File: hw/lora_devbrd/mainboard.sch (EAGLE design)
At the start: 15 parts, among them IC1 FT232RL, U1 RHF78-052

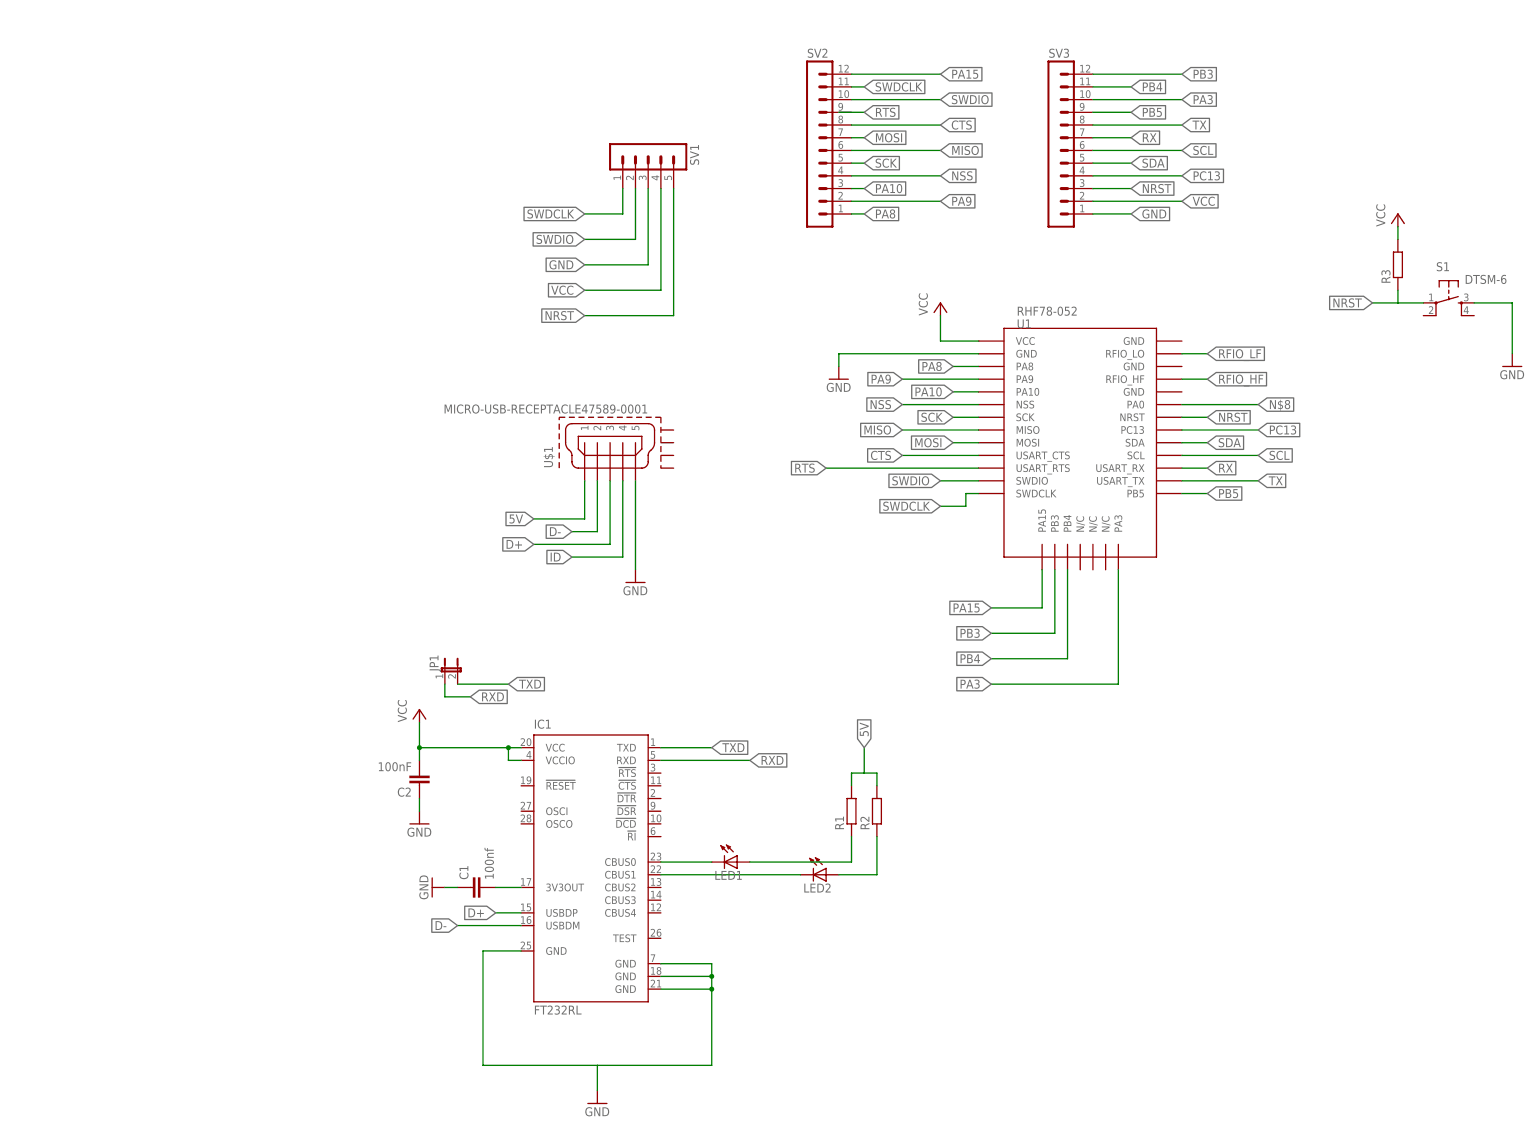
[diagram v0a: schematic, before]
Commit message: Adds LM1117
TODO:
            * trace board
            * check, check, check
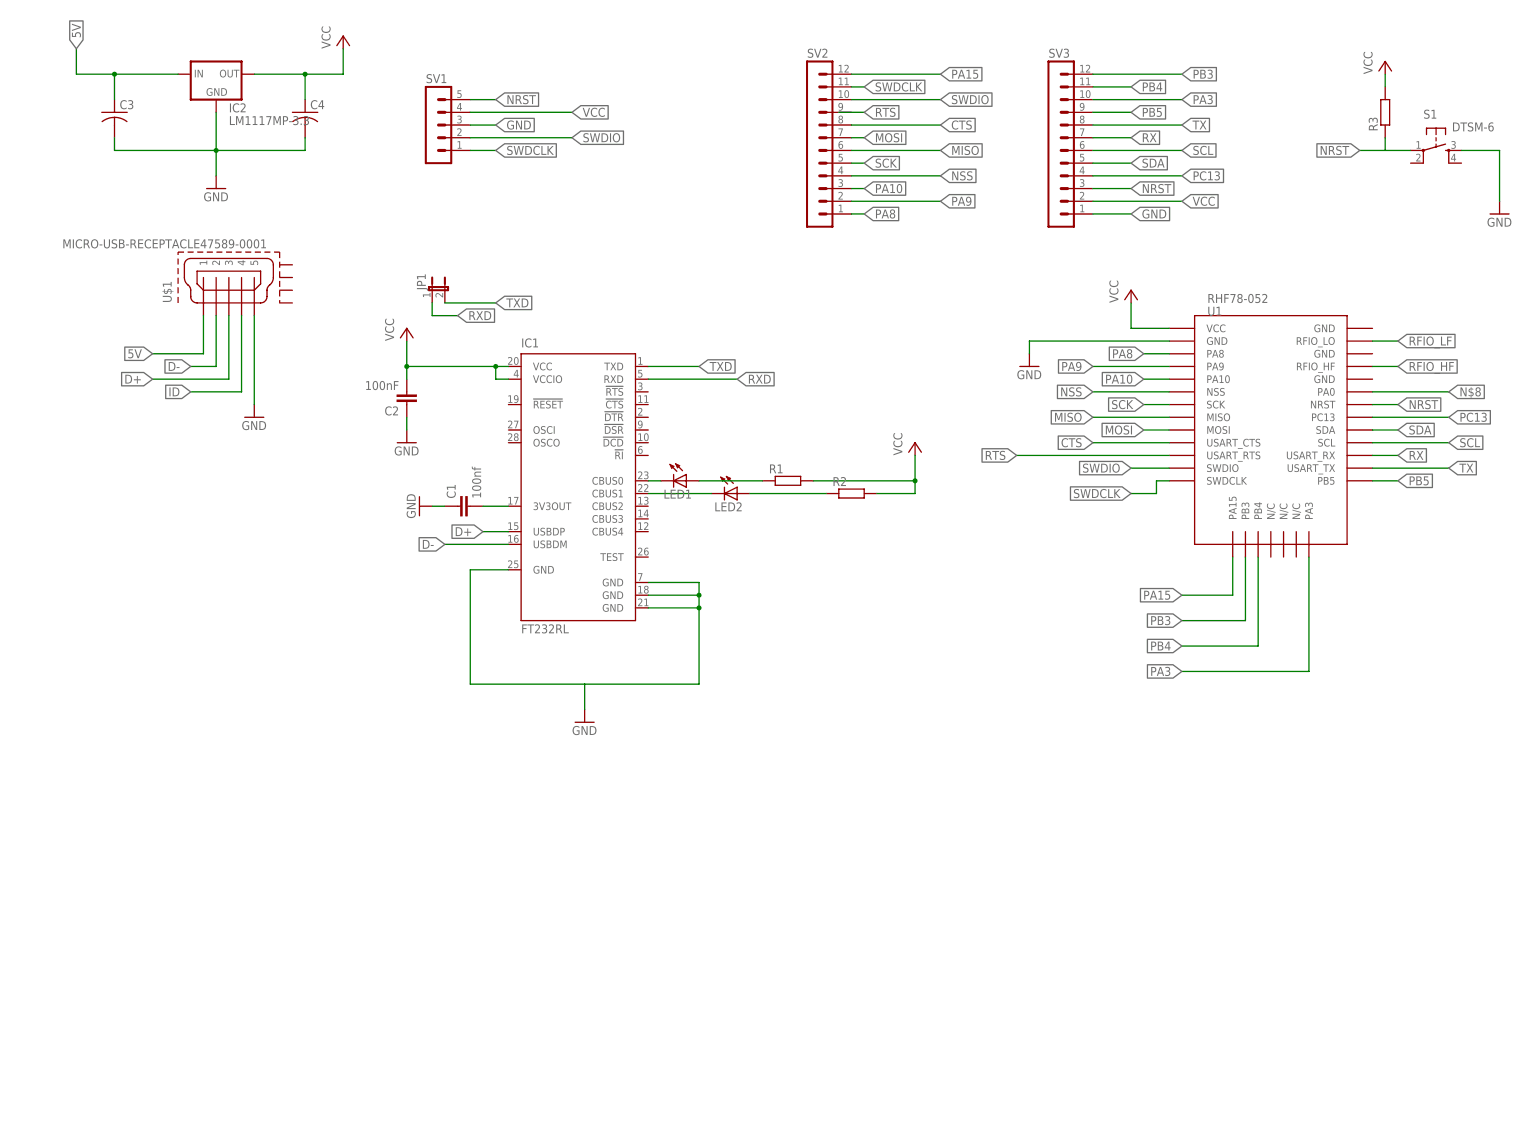
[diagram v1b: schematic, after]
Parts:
- added C3, C4: (no value), rcl:C-USC1206
- added IC2: LM1117MP-3.3, lm1117_10:LM1117MP-3.3
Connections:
- net 5V: now also C3.1, IC2.IN; no longer R1.2, R2.2
- net GND: now also C3.2, C4.2, IC2.GND
- net VCC: now also C4.1, IC2.OUT, R1.2, R2.2
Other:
- moved on the sheet: C1, C2, IC1, JP1, LED1, LED2, R1, R2, R3, S1, SV1, U$1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
